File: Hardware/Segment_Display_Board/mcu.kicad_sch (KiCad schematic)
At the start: 26 parts, among them J201 Tag Connect, J202 EXT BTN, SW201 RESET, SW202 DAY_RESET, SW203 DAY_ADV, SW204 DAY_SUB, U201 ATmega328P-A, U202 DS1307Z+, Y201 16mHz, Y202 32.768kHz

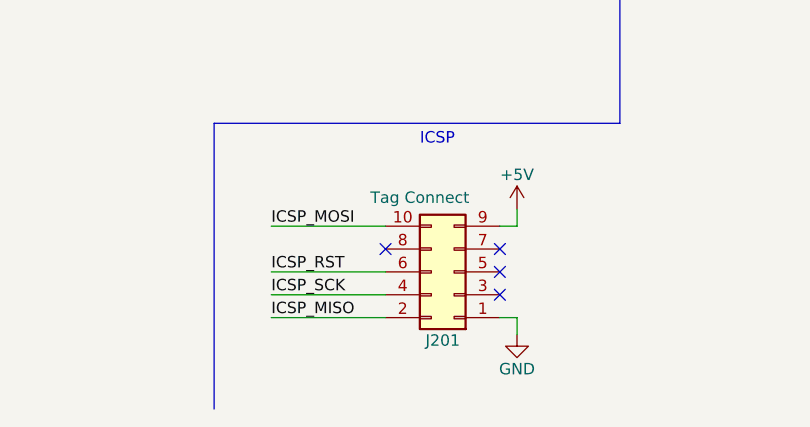
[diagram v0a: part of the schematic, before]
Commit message: Possible rewire
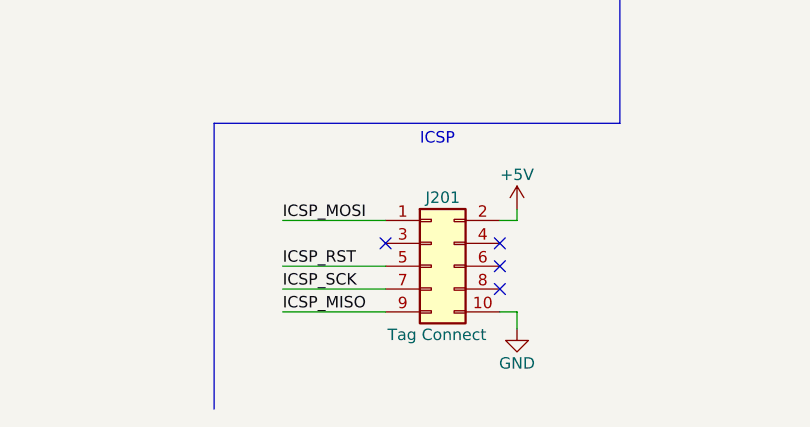
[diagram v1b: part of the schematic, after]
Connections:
- net +5V: now also J201.2 (Pin_2); no longer J201.9 (Pin_9)
- net GND: now also J201.10 (Pin_10); no longer J201.1 (Pin_1)
- net ICSP_MISO: now also J201.9 (Pin_9); no longer J201.2 (Pin_2)
- net ICSP_MOSI: now also J201.1 (Pin_1); no longer J201.10 (Pin_10)
- net ICSP_RST: now also J201.5 (Pin_5); no longer J201.6 (Pin_6)
- net ICSP_SCK: now also J201.7 (Pin_7); no longer J201.4 (Pin_4)
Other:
- moved on the sheet: J201
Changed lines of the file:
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@@
   (no_connect (at 109.855 107.315))
   (no_connect (at 109.855 81.915))
-  (no_connect (at 163.83 182.245))
   (no_connect (at 79.375 59.055))
+  (no_connect (at 163.83 181.61))
+  (no_connect (at 163.83 184.15))
   (no_connect (at 109.855 109.855))
-  (no_connect (at 163.83 179.705))
+  (no_connect (at 163.83 179.07))
   (no_connect (at 109.855 76.835))
   (no_connect (at 109.855 112.395))
   (no_connect (at 109.855 74.295))
-  (no_connect (at 151.13 179.705))
+  (no_connect (at 151.13 179.07))
   (no_connect (at 109.855 79.375))
-  (no_connect (at 163.83 184.785))
   (no_connect (at 79.375 56.515))
   (no_connect (at 243.205 50.8))
@@
     (stroke (width 0) (type default) (color 0 0 0 0))
   )
+  (wire (pts (xy 139.7 176.53) (xy 151.13 176.53))
+    (stroke (width 0) (type default) (color 0 0 0 0))
+  )
   (wire (pts (xy 134.62 88.9) (xy 111.76 88.9))
     (stroke (width 0) (type default) (color 0 0 0 0))
@@
     (stroke (width 0) (type default) (color 0 0 0 0))
   )
-  (wire (pts (xy 138.43 187.325) (xy 151.13 187.325))
-    (stroke (width 0) (type default) (color 0 0 0 0))
-  )
   (wire (pts (xy 205.74 59.69) (xy 205.74 58.42))
     (stroke (width 0) (type default) (color 0 0 0 0))
@@
     (stroke (width 0) (type default) (color 0 0 0 0))
   )
+  (wire (pts (xy 163.83 176.53) (xy 165.735 176.53))
+    (stroke (width 0) (type default) (color 0 0 0 0))
+  )
   (wire (pts (xy 75.565 51.435) (xy 75.565 53.975))
     (stroke (width 0) (type default) (color 0 0 0 0))
@@
     (stroke (width 0) (type default) (color 0 0 0 0))
   )
+  (wire (pts (xy 165.735 176.53) (xy 165.735 175.26))
+    (stroke (width 0) (type default) (color 0 0 0 0))
+  )
   (wire (pts (xy 250.19 88.9) (xy 250.19 90.17))
     (stroke (width 0) (type default) (color 0 0 0 0))
   )
+  (wire (pts (xy 139.7 186.69) (xy 151.13 186.69))
+    (stroke (width 0) (type default) (color 0 0 0 0))
+  )
   (wire (pts (xy 109.855 97.155) (xy 147.32 97.155))
     (stroke (width 0) (type default) (color 0 0 0 0))
@@
     (stroke (width 0) (type default) (color 0 0 0 0))
   )
-  (wire (pts (xy 138.43 182.245) (xy 151.13 182.245))
-    (stroke (width 0) (type default) (color 0 0 0 0))
-  )
-  (wire (pts (xy 165.735 177.165) (xy 163.83 177.165))
-    (stroke (width 0) (type default) (color 0 0 0 0))
-  )
   (wire (pts (xy 257.175 113.03) (xy 259.08 113.03))
     (stroke (width 0) (type default) (color 0 0 0 0))
@@
     (stroke (width 0) (type default) (color 0 0 0 0))
   )
+  (wire (pts (xy 139.7 181.61) (xy 151.13 181.61))
+    (stroke (width 0) (type default) (color 0 0 0 0))
+  )
   (wire (pts (xy 257.175 113.03) (xy 257.175 114.935))
     (stroke (width 0) (type default) (color 0 0 0 0))
@@
     (stroke (width 0) (type default) (color 0 0 0 0))
   )
-  (wire (pts (xy 138.43 184.785) (xy 151.13 184.785))
+  (wire (pts (xy 163.83 186.69) (xy 165.735 186.69))
     (stroke (width 0) (type default) (color 0 0 0 0))
   )
@@
     (stroke (width 0) (type default) (color 0 0 0 0))
   )
-  (wire (pts (xy 165.735 189.23) (xy 165.735 187.325))
-    (stroke (width 0) (type default) (color 0 0 0 0))
-  )
   (polyline (pts (xy 177.165 165.735) (xy 132.08 165.735))
     (stroke (width 0) (type default) (color 0 0 0 0))
@@
     (stroke (width 0) (type default) (color 0 0 0 0))
   )
-  (wire (pts (xy 165.735 187.325) (xy 163.83 187.325))
-    (stroke (width 0) (type default) (color 0 0 0 0))
-  )
   (polyline (pts (xy 177.165 12.065) (xy 177.165 165.735))
     (stroke (width 0) (type default) (color 0 0 0 0))
@@
     (stroke (width 0) (type default) (color 0 0 0 0))
   )
+  (wire (pts (xy 165.735 186.69) (xy 165.735 188.595))
+    (stroke (width 0) (type default) (color 0 0 0 0))
+  )
   (wire (pts (xy 95.885 42.545) (xy 94.615 42.545))
     (stroke (width 0) (type default) (color 0 0 0 0))
@@
     (stroke (width 0) (type default) (color 0 0 0 0))
   )
-  (wire (pts (xy 138.43 177.165) (xy 151.13 177.165))
-    (stroke (width 0) (type default) (color 0 0 0 0))
-  )
   (wire (pts (xy 271.78 144.145) (xy 271.78 146.685))
     (stroke (width 0) (type default) (color 0 0 0 0))
   )
+  (wire (pts (xy 139.7 184.15) (xy 151.13 184.15))
+    (stroke (width 0) (type default) (color 0 0 0 0))
+  )
   (wire (pts (xy 137.16 81.28) (xy 141.605 81.28))
     (stroke (width 0) (type default) (color 0 0 0 0))
@@
     (stroke (width 0) (type default) (color 0 0 0 0))
   )
-  (wire (pts (xy 165.735 175.26) (xy 165.735 177.165))
-    (stroke (width 0) (type default) (color 0 0 0 0))
-  )
   (wire (pts (xy 116.205 56.515) (xy 109.855 56.515))
     (stroke (width 0) (type default) (color 0 0 0 0))
@@
     (effects (font (size 1.27 1.27)) (justify left bottom))
   )
-  (label "ICSP_MOSI" (at 138.43 177.165 0)
+  (label "ICSP_MOSI" (at 139.7 176.53 0)
     (effects (font (size 1.27 1.27)) (justify left bottom))
   )
@@
     (effects (font (size 1.27 1.27)) (justify right bottom))
   )
-  (label "ICSP_MISO" (at 138.43 187.325 0)
+  (label "ICSP_MISO" (at 139.7 186.69 0)
     (effects (font (size 1.27 1.27)) (justify left bottom))
   )
@@
     (effects (font (size 1.27 1.27)) (justify left bottom))
   )
-  (label "ICSP_SCK" (at 138.43 184.785 0)
+  (label "ICSP_SCK" (at 139.7 184.15 0)
     (effects (font (size 1.27 1.27)) (justify left bottom))
   )
@@
     (effects (font (size 1.27 1.27)) (justify left bottom))
   )
-  (label "ICSP_RST" (at 138.43 182.245 0)
+  (label "ICSP_RST" (at 139.7 181.61 0)
     (effects (font (size 1.27 1.27)) (justify left bottom))
   )
@@
     (pin "1")
   )
-  (symbol (lib_id "Connector_Generic:Conn_02x05_Odd_Even") (at 158.75 182.245 180) (unit 1)
-    (in_bom yes) (on_board yes)
-    (property "Reference" "J201" (id 0) (at 157.48 189.865 0))
-    (property "Value" "Tag Connect" (id 1) (at 154.94 173.99 0))
-    (property "Footprint" "Connector:Tag-Connect_TC2050-IDC-FP_2x05_P1.27mm_Vertical" (id 2) (at 158.75 182.245 0)
-      (effects (font (size 1.27 1.27)) hide)
-    )
-    (property "Datasheet" "~" (id 3) (at 158.75 182.245 0)
+  (symbol (lib_id "Connector_Generic:Conn_02x05_Odd_Even") (at 156.21 181.61 0) (unit 1)
+    (in_bom yes) (on_board yes)
+    (property "Reference" "J201" (id 0) (at 157.48 173.99 0))
+    (property "Value" "Tag Connect" (id 1) (at 156.845 189.23 0))
+    (property "Footprint" "Connector:Tag-Connect_TC2050-IDC-FP_2x05_P1.27mm_Vertical" (id 2) (at 156.21 181.61 0)
+      (effects (font (size 1.27 1.27)) hide)
+    )
+    (property "Datasheet" "~" (id 3) (at 156.21 181.61 0)
       (effects (font (size 1.27 1.27)) hide)
     )
@@
     (pin "1")
   )
-  (symbol (lib_id "power:GND") (at 165.735 189.23 0) (unit 1)
-    (in_bom yes) (on_board yes)
-    (property "Reference" "#PWR0209" (id 0) (at 165.735 195.58 0)
-      (effects (font (size 1.27 1.27)) hide)
-    )
-    (property "Value" "GND" (id 1) (at 165.735 193.04 0))
-    (property "Footprint" "" (id 2) (at 165.735 189.23 0)
-      (effects (font (size 1.27 1.27)) hide)
-    )
-    (property "Datasheet" "" (id 3) (at 165.735 189.23 0)
-      (effects (font (size 1.27 1.27)) hide)
-    )
+  (symbol (lib_id "power:GND") (at 165.735 188.595 0) (unit 1)
+    (in_bom yes) (on_board yes)
+    (property "Reference" "#PWR0209" (id 0) (at 165.735 194.945 0)
+      (effects (font (size 1.27 1.27)) hide)
+    )
+    (property "Value" "GND" (id 1) (at 165.735 192.405 0))
+    (property "Footprint" "" (id 2) (at 165.735 188.595 0)
+      (effects (font (size 1.27 1.27)) hide)
+    )
+    (property "Datasheet" "" (id 3) (at 165.735 188.595 0)
+      (effects (font (size 1.27 1.27)) hide)
+    )
